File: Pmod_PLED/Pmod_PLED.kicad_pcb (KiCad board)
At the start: 2 copper layers, 75.8 x 20 mm, 7 parts, among them IC1 TBD62064APG, IC2 LM2940T-5.0, J1 Barrel_Jack_Switch, J2 Conn_01x06_Pin, J3 Conn_01x03_Pin

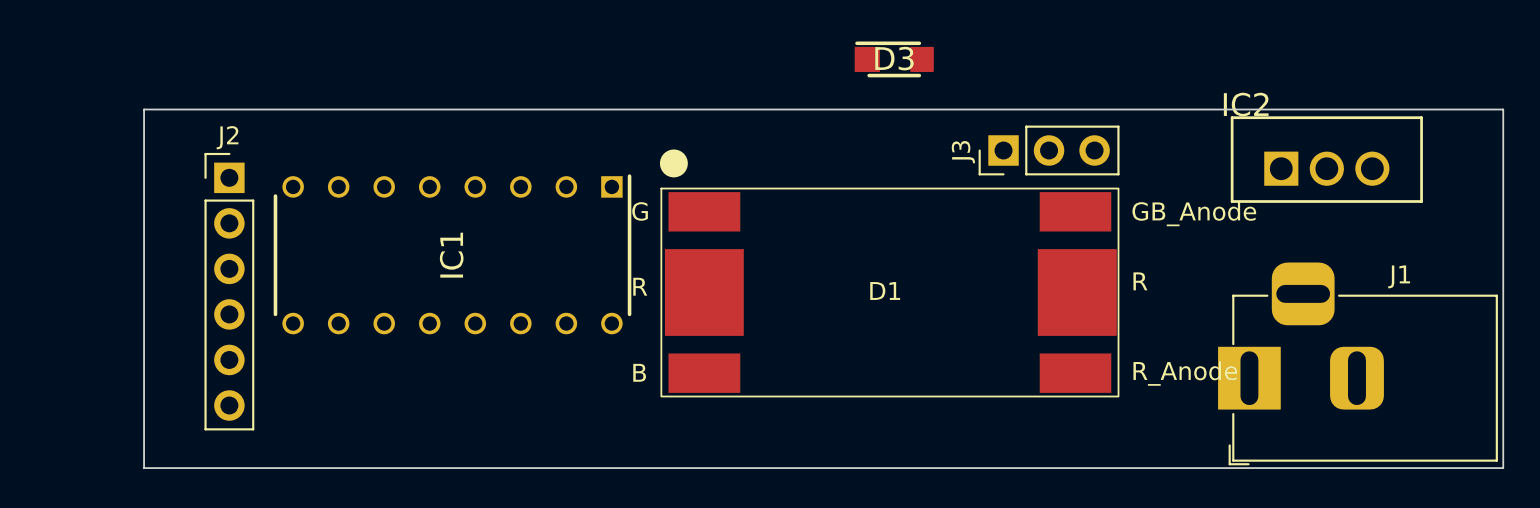
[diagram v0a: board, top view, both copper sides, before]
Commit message: 30
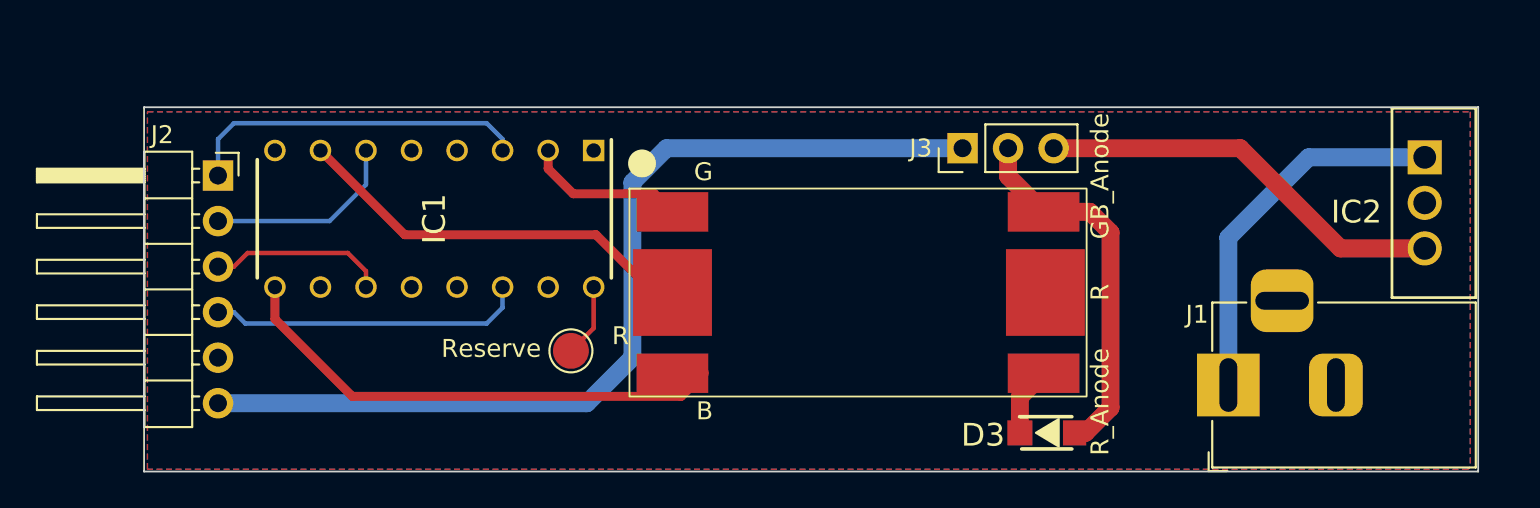
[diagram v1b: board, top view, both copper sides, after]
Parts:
- added Reserve: TestPoint, TestPoint:TestPoint_Pad_D2.0mm, F.Cu at (112.3, 89.7)
- D1: value EP204K-150G1R1B1-CA -> [EP204K-150G1R1B1-CA]
- J2: footprint Connector_PinHeader_2.54mm:PinHeader_1x06_P2.54mm_Vertical -> Library:Pmod6
- moved D3 22.5 mm to (138.8, 94.2)
- moved J2 9.40 mm to (83.8, 79.9)
- moved IC2 6.73 mm to (160.9, 83.9), turned to -90 degrees
- moved J3 2.29 mm to (134.1, 78.4)
- moved IC1 2.27 mm to (104.6, 82.3)
- moved D1 1.78 mm to (128.3, 86.4)
- moved J1 1.23 mm to (148.9, 91.6)
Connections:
- D1 pad 2: unconnected-(D1-RK-Pad2) -> Net-(IC1-O2)
- D1 pad 5: Net-(D1-A) -> unconnected-(D1-RK-Pad5)
- D1 pad 6: Net-(D1-A) -> /Anode
- D3 pad 2: Net-(D1-A) -> /Anode
- IC1 pad 14: GND -> Net-(IC1-I4)
- IC1 pad 16: unconnected-(IC1-O4-Pad16) -> Net-(IC1-O4)
- IC1 pad 7: unconnected-(IC1-O2-Pad7) -> Net-(IC1-O2)
- J2 pad 4: unconnected-(J2-Pin_4-Pad4) -> Net-(IC1-I4)
- J3 pad 2: Net-(D1-A) -> /Anode
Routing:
- net VCC: track 0.00 -> 53.1 mm
- net Net-(D1-BK): track 0.00 -> 28.1 mm
- net /ExVcc: track 0.00 -> 23.0 mm
- net Net-(IC1-O2): track 0.00 -> 22.9 mm
- net Net-(IC2-IN): track 0.00 -> 21.0 mm
- net /Anode: track 0.00 -> 20.9 mm
- net Net-(IC1-I1): track 0.00 -> 19.3 mm
- net Net-(IC1-I4): track 0.00 -> 17.6 mm
- net Net-(IC1-I2): track 0.00 -> 11.0 mm
- net Net-(IC1-I3): track 0.00 -> 9.88 mm
- net Net-(D1-GK): track 0.00 -> 8.95 mm
- net Net-(IC1-O4): track 0.00 -> 4.08 mm
- net Net-(D1-RA): track 0.00 -> 3.87 mm
- added copper zone on B.Cu, net GND
- added copper zone on F.Cu, net GND
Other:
- board size 75.8 x 20 mm -> 74.4 x 20.3 mm
- board text added: "[EP204K- 150G1R1B1-CA]"
